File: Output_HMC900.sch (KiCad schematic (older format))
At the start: 5 parts

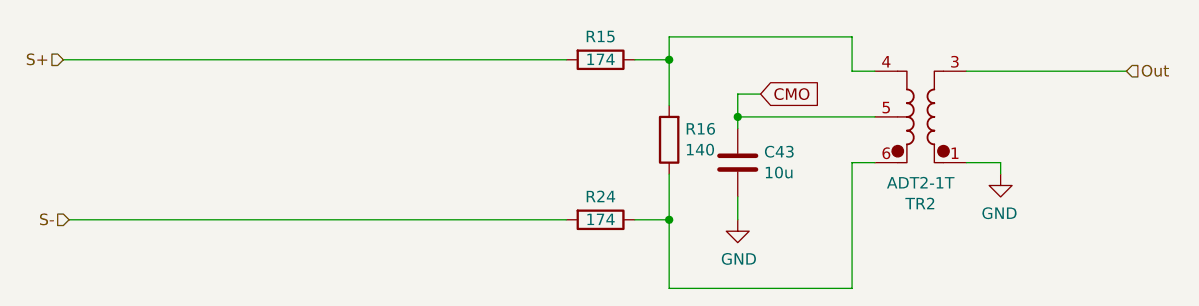
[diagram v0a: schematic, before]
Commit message: Changed input transformer reference to 2.5v
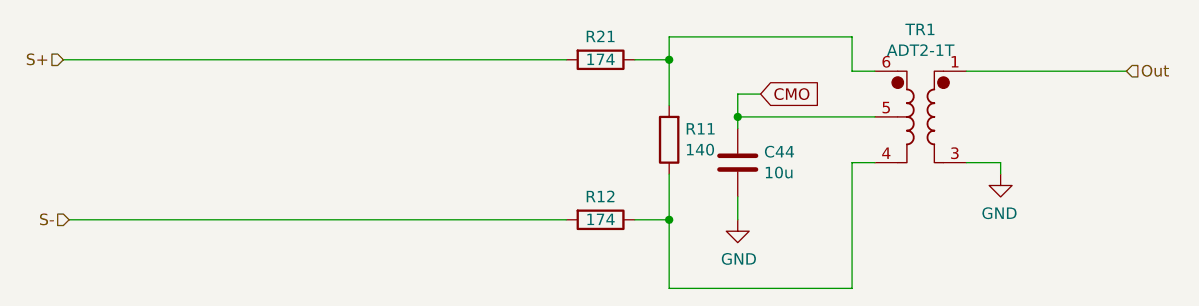
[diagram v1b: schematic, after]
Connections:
- net GND: now also TR1.3; no longer TR1.1
- net Out: now also TR1.1; no longer TR1.3
- net at R11.1, R12.1: now also TR1.4; no longer TR1.6
- net at R11.2, R21.1: now also TR1.6; no longer TR1.4
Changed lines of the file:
@@
 $Descr A4 11693 8268
 encoding utf-8
-Sheet 6 7
+Sheet 3 7
 Title ""
 Date ""
@@
 AR Path="/60D21B6E/6160D475/614E552D" Ref="R16"  Part="1"
 AR Path="/60D21B6E/60F5ADAC/614E552D" Ref="R16"  Part="1"
-F 0 "R16" H 5980 3254 50  0000 R CNN
+F 0 "R11" H 5980 3254 50  0000 R CNN
 F 1 "140" H 5980 3345 50  0000 R CNN
 F 2 "Resistor_SMD:R_0603_1608Metric_Pad0.98x0.95mm_HandSolder" V 5980 3300 50  0001 C CNN
@@
 AR Path="/60D21B6E/6160D475/614E5533" Ref="R24"  Part="1"
 AR Path="/60D21B6E/60F5ADAC/614E5533" Ref="R15"  Part="1"
-F 0 "R15" V 5650 2950 50  0000 C CNN
+F 0 "R21" V 5650 2950 50  0000 C CNN
 F 1 "174" V 5750 2950 50  0000 C CNN
 F 2 "Resistor_SMD:R_0603_1608Metric_Pad0.98x0.95mm_HandSolder" V 5680 2950 50  0001 C CNN
@@
 AR Path="/60D21B6E/6160D475/614E5539" Ref="C43"  Part="1"
 AR Path="/60D21B6E/60F5ADAC/614E5539" Ref="C43"  Part="1"
-F 0 "C43" H 6465 3446 50  0000 L CNN
+F 0 "C44" H 6465 3446 50  0000 L CNN
 F 1 "10u" H 6465 3355 50  0000 L CNN
 F 2 "Capacitor_SMD:C_0603_1608Metric_Pad1.08x0.95mm_HandSolder" H 6388 3250 50  0001 C CNN
@@
 AR Path="/60D21B6E/6160D475/614E55C8" Ref="R15"  Part="1"
 AR Path="/60D21B6E/60F5ADAC/614E55C8" Ref="R24"  Part="1"
-F 0 "R24" V 5650 3650 50  0000 C CNN
+F 0 "R12" V 5650 3650 50  0000 C CNN
 F 1 "174" V 5750 3650 50  0000 C CNN
 F 2 "Resistor_SMD:R_0603_1608Metric_Pad0.98x0.95mm_HandSolder" V 5680 3650 50  0001 C CNN
@@
 AR Path="/60D21B6E/6160D475/614E5545" Ref="TR2"  Part="1"
 AR Path="/60D21B6E/60F5ADAC/614E5545" Ref="TR2"  Part="1"
-F 0 "TR2" H 7150 3581 50  0000 C CNN
+F 0 "TR1" H 7150 3581 50  0000 C CNN
 F 1 "ADT2-1T" H 7150 3490 50  0000 C CNN
 F 2 "RF_Mini-Circuits:Mini-Circuits_CD542_H2.84mm" H 7150 2850 50  0001 C CNN
 F 3 "https://www.minicircuits.com/pdfs/ADT2-1T+.pdf" H 7150 3200 50  0001 C CNN
 	1    7150 3200
-	-1   0    0    1
+	-1   0    0    -1
 $EndComp
 Connection ~ 6350 3200

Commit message: Straitened things before restarting routing
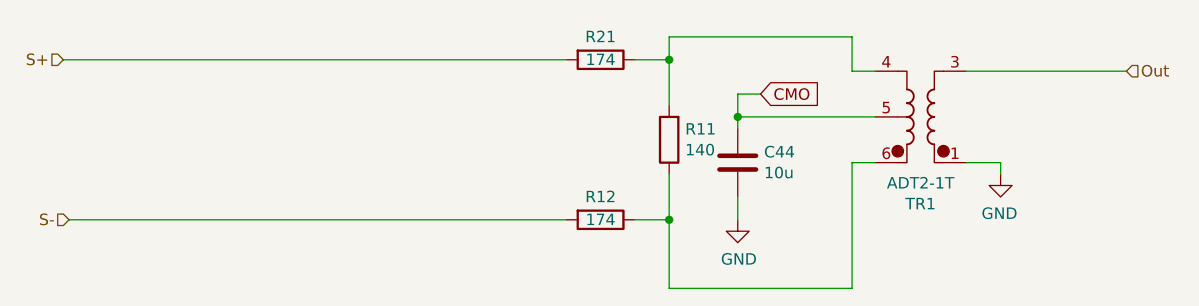
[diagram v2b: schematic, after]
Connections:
- net GND: now also TR1.1; no longer TR1.3
- net Out: now also TR1.3; no longer TR1.1
- net at R11.1, R12.1: now also TR1.6; no longer TR1.4
- net at R11.2, R21.1: now also TR1.4; no longer TR1.6
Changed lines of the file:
@@
 AR Path="/60D21B6E/6160D475/614E557C" Ref="#PWR0140"  Part="1"
 AR Path="/60D21B6E/60F5ADAC/614E557C" Ref="#PWR0139"  Part="1"
-F 0 "#PWR0139" H 6350 3400 50  0001 C CNN
+F 0 "#PWR0128" H 6350 3400 50  0001 C CNN
 F 1 "GND" H 6355 3477 50  0000 C CNN
 F 2 "" H 6350 3650 50  0001 C CNN
@@
 AR Path="/60D21B6E/6160D475/614E5583" Ref="#PWR0142"  Part="1"
 AR Path="/60D21B6E/60F5ADAC/614E5583" Ref="#PWR0140"  Part="1"
-F 0 "#PWR0140" H 7500 3200 50  0001 C CNN
+F 0 "#PWR0130" H 7500 3200 50  0001 C CNN
 F 1 "GND" H 7505 3277 50  0000 C CNN
 F 2 "" H 7500 3450 50  0001 C CNN
@@
 F 3 "https://www.minicircuits.com/pdfs/ADT2-1T+.pdf" H 7150 3200 50  0001 C CNN
 	1    7150 3200
-	-1   0    0    -1
+	-1   0    0    1
 $EndComp
 Connection ~ 6350 3200

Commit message: Made it so there was only one output and change the SMA (to a sourceable one)
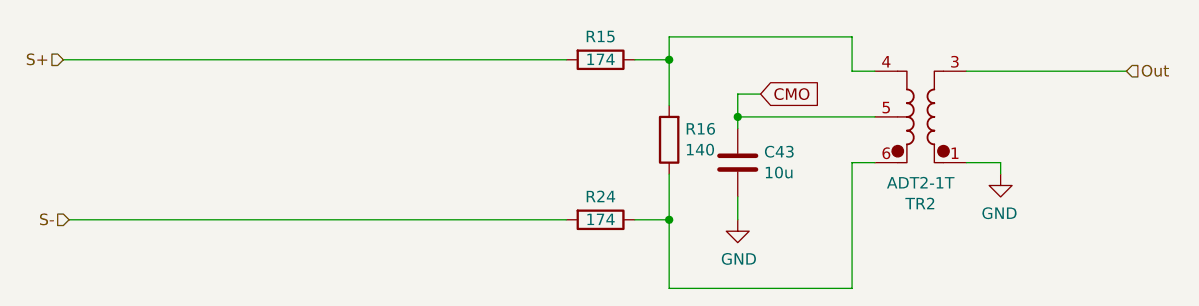
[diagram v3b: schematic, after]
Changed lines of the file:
@@
 $Descr A4 11693 8268
 encoding utf-8
-Sheet 3 7
+Sheet 6 7
 Title ""
 Date ""
@@
 AR Path="/60D21B6E/6160D475/614E552D" Ref="R16"  Part="1"
 AR Path="/60D21B6E/60F5ADAC/614E552D" Ref="R16"  Part="1"
-F 0 "R11" H 5980 3254 50  0000 R CNN
+F 0 "R16" H 5980 3254 50  0000 R CNN
 F 1 "140" H 5980 3345 50  0000 R CNN
 F 2 "Resistor_SMD:R_0603_1608Metric_Pad0.98x0.95mm_HandSolder" V 5980 3300 50  0001 C CNN
@@
 AR Path="/60D21B6E/6160D475/614E5533" Ref="R24"  Part="1"
 AR Path="/60D21B6E/60F5ADAC/614E5533" Ref="R15"  Part="1"
-F 0 "R21" V 5650 2950 50  0000 C CNN
+F 0 "R15" V 5650 2950 50  0000 C CNN
 F 1 "174" V 5750 2950 50  0000 C CNN
 F 2 "Resistor_SMD:R_0603_1608Metric_Pad0.98x0.95mm_HandSolder" V 5680 2950 50  0001 C CNN
@@
 AR Path="/60D21B6E/6160D475/614E5539" Ref="C43"  Part="1"
 AR Path="/60D21B6E/60F5ADAC/614E5539" Ref="C43"  Part="1"
-F 0 "C44" H 6465 3446 50  0000 L CNN
+F 0 "C43" H 6465 3446 50  0000 L CNN
 F 1 "10u" H 6465 3355 50  0000 L CNN
 F 2 "Capacitor_SMD:C_0603_1608Metric_Pad1.08x0.95mm_HandSolder" H 6388 3250 50  0001 C CNN
@@
 AR Path="/60D21B6E/6160D475/614E557C" Ref="#PWR0140"  Part="1"
 AR Path="/60D21B6E/60F5ADAC/614E557C" Ref="#PWR0139"  Part="1"
-F 0 "#PWR0128" H 6350 3400 50  0001 C CNN
+F 0 "#PWR0139" H 6350 3400 50  0001 C CNN
 F 1 "GND" H 6355 3477 50  0000 C CNN
 F 2 "" H 6350 3650 50  0001 C CNN
@@
 AR Path="/60D21B6E/6160D475/614E55C8" Ref="R15"  Part="1"
 AR Path="/60D21B6E/60F5ADAC/614E55C8" Ref="R24"  Part="1"
-F 0 "R12" V 5650 3650 50  0000 C CNN
+F 0 "R24" V 5650 3650 50  0000 C CNN
 F 1 "174" V 5750 3650 50  0000 C CNN
 F 2 "Resistor_SMD:R_0603_1608Metric_Pad0.98x0.95mm_HandSolder" V 5680 3650 50  0001 C CNN
@@
 AR Path="/60D21B6E/6160D475/614E5583" Ref="#PWR0142"  Part="1"
 AR Path="/60D21B6E/60F5ADAC/614E5583" Ref="#PWR0140"  Part="1"
-F 0 "#PWR0130" H 7500 3200 50  0001 C CNN
+F 0 "#PWR0140" H 7500 3200 50  0001 C CNN
 F 1 "GND" H 7505 3277 50  0000 C CNN
 F 2 "" H 7500 3450 50  0001 C CNN
@@
 AR Path="/60D21B6E/6160D475/614E5545" Ref="TR2"  Part="1"
 AR Path="/60D21B6E/60F5ADAC/614E5545" Ref="TR2"  Part="1"
-F 0 "TR1" H 7150 3581 50  0000 C CNN
+F 0 "TR2" H 7150 3581 50  0000 C CNN
 F 1 "ADT2-1T" H 7150 3490 50  0000 C CNN
 F 2 "RF_Mini-Circuits:Mini-Circuits_CD542_H2.84mm" H 7150 2850 50  0001 C CNN
